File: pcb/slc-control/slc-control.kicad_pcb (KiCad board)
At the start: 4 copper layers, 99 x 45 mm, 95 parts, among them J1 USB_C_Receptacle_USB2.0_16P, J2 Conn_01x02_Socket, J3 Conn_01x02_Socket, J4 Conn_01x02_Socket, J5 Conn_01x02_Socket, J6 Conn_Coaxial, J7 Conn_ARM_SWD_TagConnect_TC203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, J8 Conn_01x07_Pin, Q3 AO3400A, Q4 AO3401A, Q5 AO3400A, Q6 AO3400A, Q7 Q_Dual_PMOS_S1G1S2G2D2D2D1D1, Q8 AO3400A, Q9 Q_Dual_PMOS_S1G1S2G2D2D2D1D1, SW1 SW_Push, SW2 SW_Push, SW3 SW_Push, SW4 SW_Push, U1 TPS5430DDA, U2 SRV05-4, U3 AMS1117-3.3, U4 QMC5883L, U5 AT24CS32-SSHM, U6 LPS22HH, U7 STM32G431CBTx, U8 GPS02-UBX, Y1 16MHz

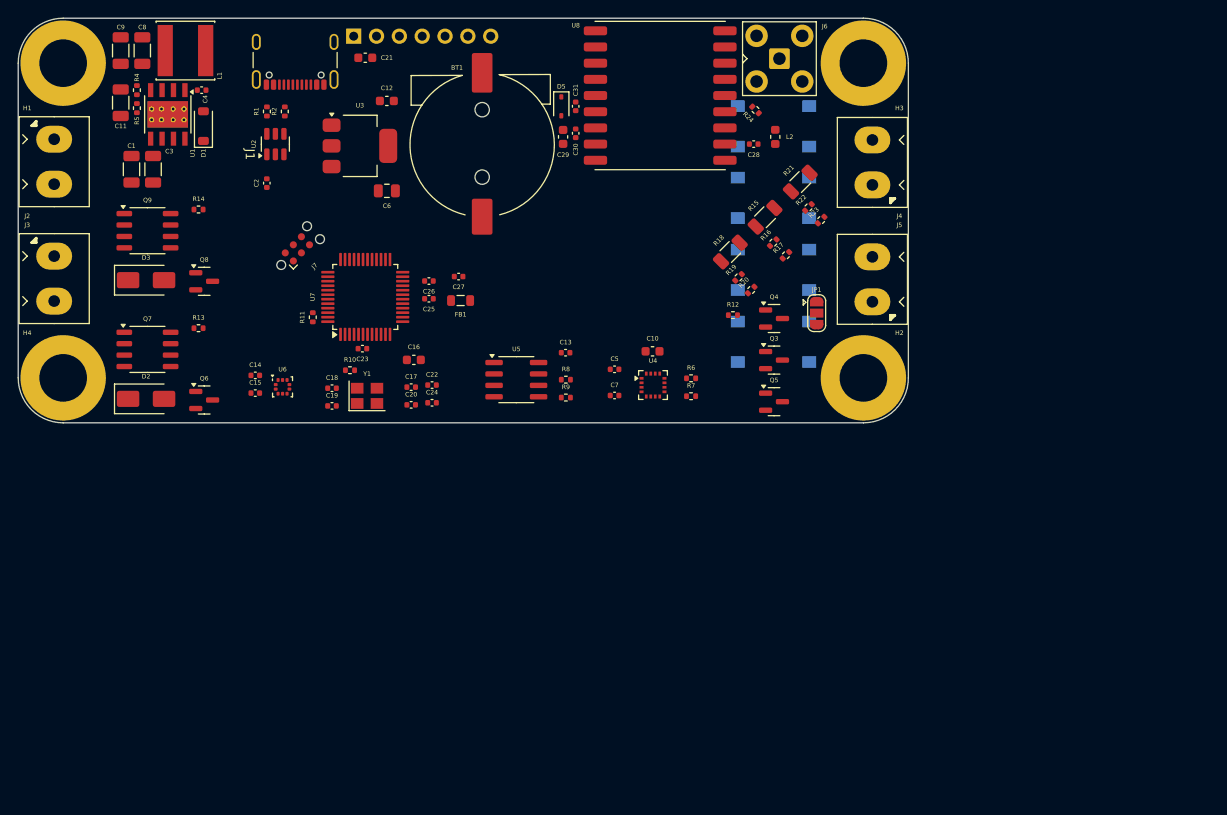
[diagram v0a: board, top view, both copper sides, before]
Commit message: Finish layout
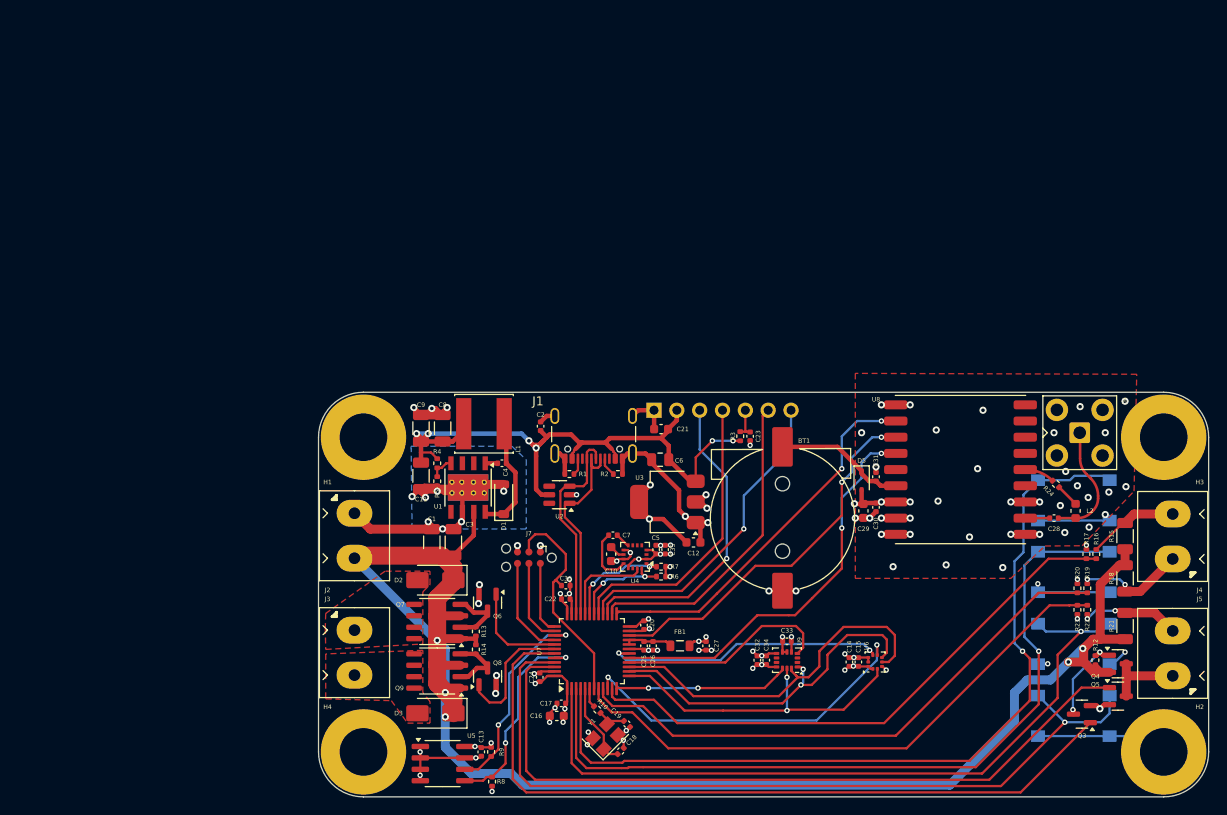
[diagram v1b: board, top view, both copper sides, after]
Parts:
- removed JP1: SolderJumper_3_Open, Jumper:SolderJumper-3_P1.3mm_Open_RoundedPad1.0x1.5mm
- removed R11: 10k, Resistor_SMD:R_0402_1005Metric
- added C32: 2u2, Capacitor_SMD:C_0402_1005Metric, F.Cu at (107.2, 126.4)
- added C33: 100n, Capacitor_SMD:C_0402_1005Metric, F.Cu at (110.5, 124.3)
- added C34: 100n, Capacitor_SMD:C_0402_1005Metric, F.Cu at (108.2, 126.4)
- added C35: 2u2, Capacitor_SMD:C_0402_1005Metric, F.Cu at (96.9, 114.1)
- added C36: 100n, Capacitor_SMD:C_0402_1005Metric, F.Cu at (85.9, 118.1)
- added R3: 33k, Resistor_SMD:R_0402_1005Metric, F.Cu at (105.3, 101.5)
- added U9: ICM-42688-P, Package_LGA:LGA-14_3x2.5mm_P0.5mm_LayoutBorder3x4y, F.Cu at (110.5, 126.4)
- moved C15 73.4 mm to (118.4, 126.6), turned to 90 degrees
- moved C14 73.4 mm to (117.4, 126.6), turned to 90 degrees
- moved U6 72.7 mm to (120.3, 126.6), turned to 90 degrees
- moved R21 61.2 mm to (148.1, 122.6), turned to 90 degrees
- moved C12 59.8 mm to (100.1, 113.3)
- moved Q9 58.6 mm to (71.6, 127.6), turned to 180 degrees
- moved D3 57.9 mm to (71.4, 132.3), turned to 180 degrees
- moved R14 57.8 mm to (75.9, 125.2), turned to -90 degrees
- moved R18 57.0 mm to (148.1, 117.3), turned to -90 degrees
- moved R12 55.7 mm to (144.8, 126.4), turned to 90 degrees
- moved R2 54.8 mm to (91.7, 105.7), turned to 0 degrees
- moved R22 54.4 mm to (143.9, 120.8), turned to 90 degrees
- moved Q4 54.2 mm to (147.3, 126.8)
- moved Q8 54.1 mm to (77.2, 128.2), turned to 90 degrees
- moved C8 53.7 mm to (72.2, 100.6)
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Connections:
- C18 pad 2: /XTALO -> /XTALI
- C23 pad 1: /RST -> /RES
- C25 pad 1: +3VA3 -> +3V3A
- C26 pad 1: +3VA3 -> +3V3A
- FB1 pad 1: +3VA3 -> +3V3A
- J5 pad 1: Net-(J5-Pin_1) -> /REP
- J8 pad 3: /SCK -> /SDK
- J8 pad 4: /MOSI -> /SDI
- R10 pad 2: /XTALI -> /XTALO
- U7 pad 10: unconnected-(U7-PA2-Pad10) -> /CSP
- U7 pad 11: unconnected-(U7-PA3-Pad11) -> /SIG1
- U7 pad 12: unconnected-(U7-PA4-Pad12) -> /CSG
- U7 pad 13: unconnected-(U7-PA5-Pad13) -> /SCK
- U7 pad 14: unconnected-(U7-PA6-Pad14) -> /MISO
- U7 pad 15: unconnected-(U7-PA7-Pad15) -> /MOSI
- U7 pad 16: unconnected-(U7-PB0-Pad16) -> /INTG1
- U7 pad 17: unconnected-(U7-PB1-Pad17) -> /PPS
- U7 pad 18: unconnected-(U7-PB2-Pad18) -> /DRDYP
- U7 pad 2: unconnected-(U7-PC13-Pad2) -> /BTN3
- U7 pad 20: +3V3 -> +3V3A
- U7 pad 21: +3VA3 -> +3V3A
- U7 pad 22: unconnected-(U7-PB10-Pad22) -> /GTX
- U7 pad 25: unconnected-(U7-PB11-Pad25) -> /GRX
- U7 pad 26: unconnected-(U7-PB12-Pad26) -> /DC
- U7 pad 27: unconnected-(U7-PB13-Pad27) -> /SDK
- U7 pad 28: unconnected-(U7-PB14-Pad28) -> /CSD
- U7 pad 29: unconnected-(U7-PB15-Pad29) -> /SDI
- U7 pad 3: unconnected-(U7-PC14-Pad3) -> /BTN2
- U7 pad 30: unconnected-(U7-PA8-Pad30) -> /SDAM
- U7 pad 31: unconnected-(U7-PA9-Pad31) -> /SCLM
- U7 pad 32: unconnected-(U7-PA10-Pad32) -> /DRDYM
- U7 pad 39: unconnected-(U7-PA15-Pad39) -> /SCLE
- U7 pad 4: unconnected-(U7-PC15-Pad4) -> /BTN1
- U7 pad 41: unconnected-(U7-PB4-Pad41) -> /DRV1
- U7 pad 42: unconnected-(U7-PB5-Pad42) -> /DRV2
- U7 pad 43: unconnected-(U7-PB6-Pad43) -> /REPH
- U7 pad 44: unconnected-(U7-PB7-Pad44) -> /SDAE
- U7 pad 45: /BOOT0 -> /BTN4
- U7 pad 46: unconnected-(U7-PB9-Pad46) -> /REPL
- U7 pad 8: unconnected-(U7-PA0-Pad8) -> /SIG3
- U7 pad 9: unconnected-(U7-PA1-Pad9) -> /SIG2
- U8 pad 18: /GRST -> +3V3
- Y1 pad 1: /XTALO -> /XTALI
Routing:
- net +12V: track 0.00 -> 180.8 mm, vias 0 -> 5
- net GND: track 0.00 -> 176.4 mm, vias 0 -> 86
- net /BTN1: track 0.00 -> 95.0 mm, vias 0 -> 1
- net /BTN4: track 0.00 -> 91.6 mm, vias 0 -> 1
- net /BTN2: track 0.00 -> 88.8 mm, vias 0 -> 1
- net /REPH: track 0.00 -> 85.9 mm
- net /REPL: track 0.00 -> 83.9 mm
- net /BTN3: track 0.00 -> 83.4 mm, vias 0 -> 1
- net +5V: track 0.00 -> 74.5 mm, vias 0 -> 6
- net +3V3: track 0.00 -> 65.7 mm, vias 0 -> 32
- net /SIG3: track 0.00 -> 64.4 mm
- net /SIG1: track 0.00 -> 63.5 mm
- net /SIG2: track 0.00 -> 63.1 mm
- net /PPS: track 0.00 -> 44.7 mm, vias 0 -> 2
- net /GRX: track 0.00 -> 42.0 mm, vias 0 -> 2
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- added copper zone on In2.Cu, net +3V3
- added copper zone on F.Cu, net /OUT1
- added copper zone on F.Cu, net /OUT2
- added copper zone on B.Cu, net GND
- added copper zone on F.Cu, net GND
- added copper zone on In1.Cu, net GND
